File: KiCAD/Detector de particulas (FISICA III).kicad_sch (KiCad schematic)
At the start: 22 parts, among them J1 Conn_01x02_Female, J2 Conn_01x02_Female, U1 OPA2134PA

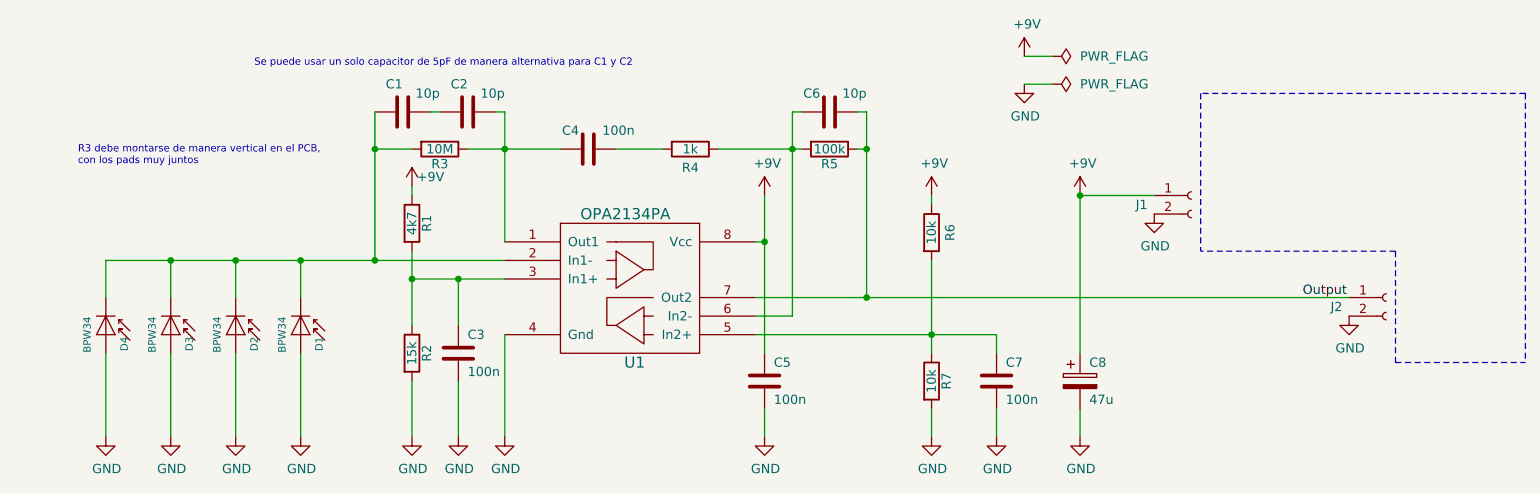
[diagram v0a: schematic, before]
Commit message: nuevo pcb
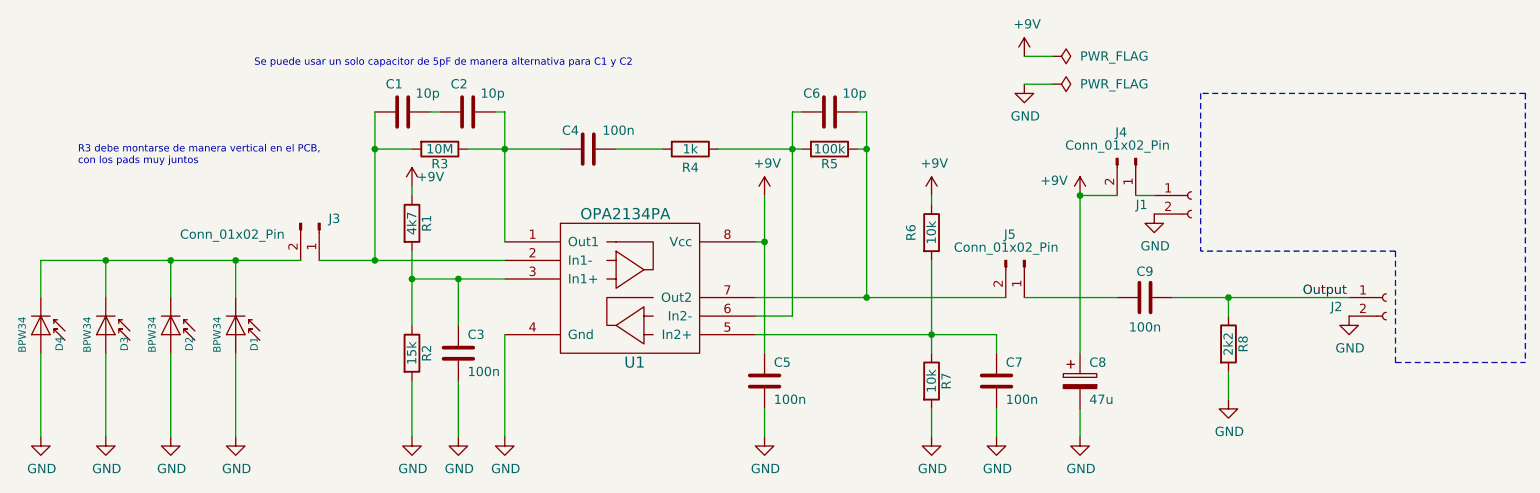
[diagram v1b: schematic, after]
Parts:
- added C9: 100n, Capacitor_THT:C_Disc_D3.0mm_W1.6mm_P2.50mm, symbol Device:C
- added J3, J4, J5: Conn_01x02_Pin, Connector_PinHeader_2.54mm:PinHeader_1x02_P2.54mm_Vertical, symbol Connector:Conn_01x02_Pin
- added R8: 2k2, Resistor_THT:R_Axial_DIN0207_L6.3mm_D2.5mm_P7.62mm_Horizontal, symbol Device:R
- R3: footprint Resistor_THT:R_Axial_DIN0204_L3.6mm_D1.6mm_P7.62mm_Horizontal -> Resistor_THT:R_Axial_DIN0309_L9.0mm_D3.2mm_P2.54mm_Vertical
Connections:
- net +9V: now also J4.2 (Pin_2); no longer J1.1 (Pin_1)
- net GND: now also R8.2
- net Output: now also C9.2, R8.1; no longer C6.2, R5.1, U1.7 (Out2)
- net at D1.1 (K), D2.1 (K), D3.1 (K)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: now also J3.2 (Pin_2); no longer C1.1, R3.2, U1.2 (In1-)
- new net: C1.1, J3.1 (Pin_1), R3.2, U1.2 (In1-)
- new net: C6.2, J5.2 (Pin_2), R5.1, U1.7 (Out2)
- new net: J1.1 (Pin_1), J4.1 (Pin_1)
- new net: C9.1, J5.1 (Pin_1)
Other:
- moved on the sheet: D1, D2, D3, D4

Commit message: primera version terminada
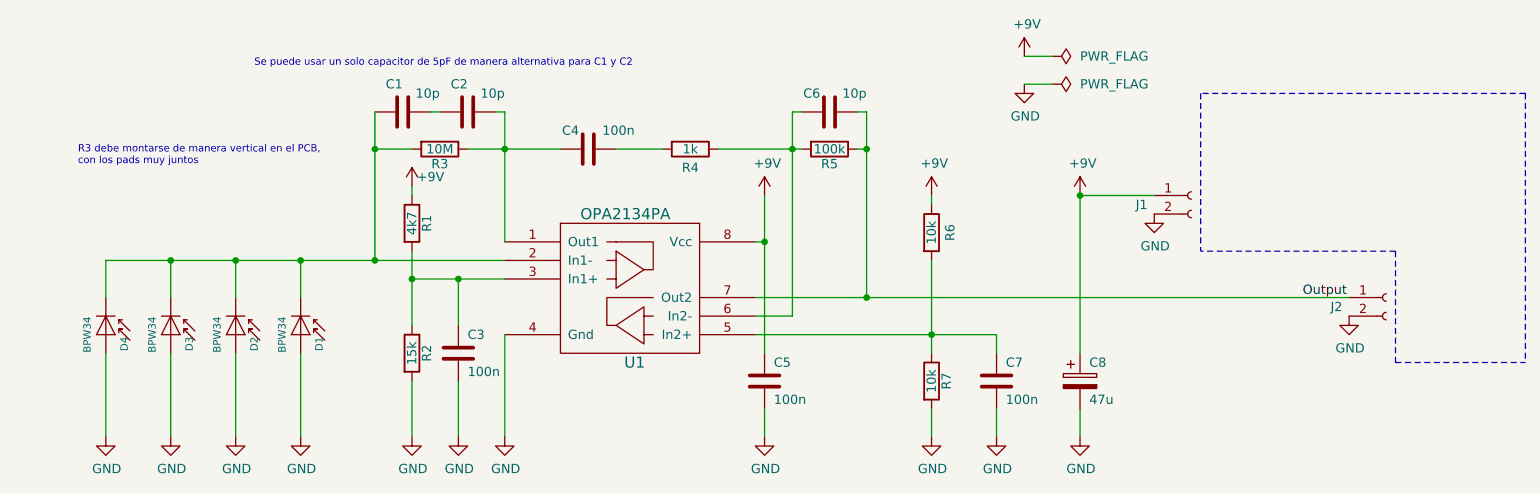
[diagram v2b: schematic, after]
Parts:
- removed C9: 100n, Capacitor_THT:C_Disc_D3.0mm_W1.6mm_P2.50mm, symbol Device:C
- removed J3, J4, J5: Conn_01x02_Pin, Connector_PinHeader_2.54mm:PinHeader_1x02_P2.54mm_Vertical, symbol Connector:Conn_01x02_Pin
- removed R8: 2k2, Resistor_THT:R_Axial_DIN0207_L6.3mm_D2.5mm_P7.62mm_Horizontal, symbol Device:R
- R3: footprint Resistor_THT:R_Axial_DIN0309_L9.0mm_D3.2mm_P2.54mm_Vertical -> Resistor_THT:R_Axial_DIN0204_L3.6mm_D1.6mm_P7.62mm_Horizontal
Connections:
- net +9V: now also J1.1 (Pin_1)
- net Output: now also C6.2, R5.1, U1.7 (Out2)
- net at C1.1, R3.2, U1.2 (In1-): now also D1.1 (K), D2.1 (K), D3.1 (K), D4.1 (K)
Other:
- moved on the sheet: D1, D2, D3, D4
